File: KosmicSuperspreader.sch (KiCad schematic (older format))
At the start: 27 parts

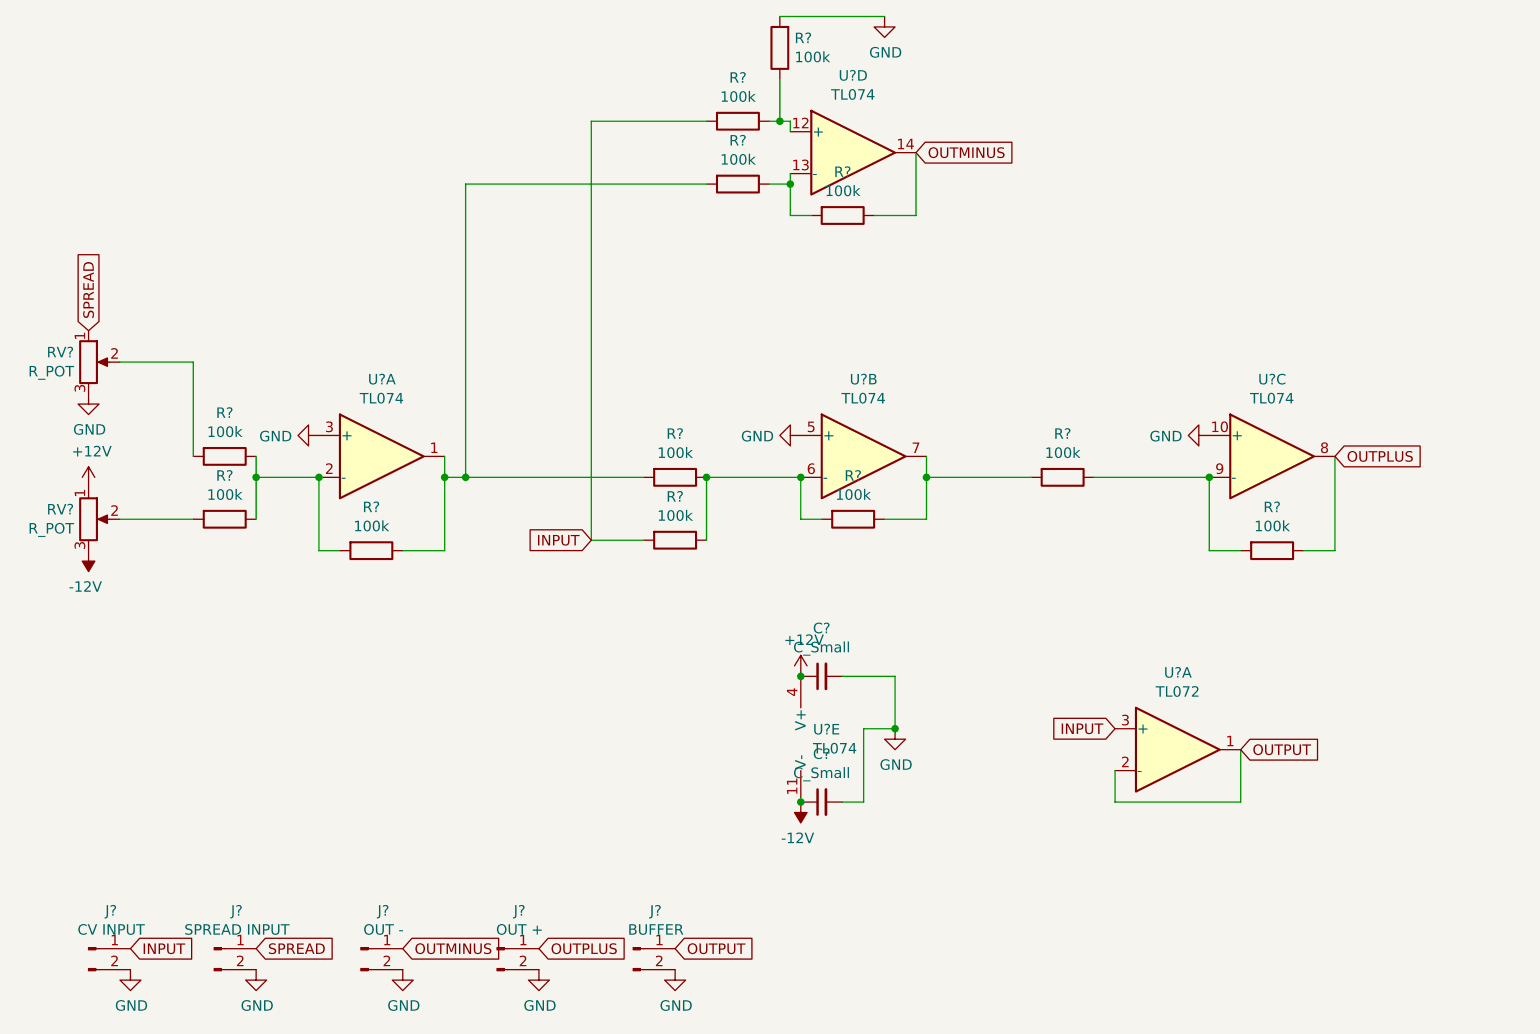
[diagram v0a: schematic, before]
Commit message: Power...
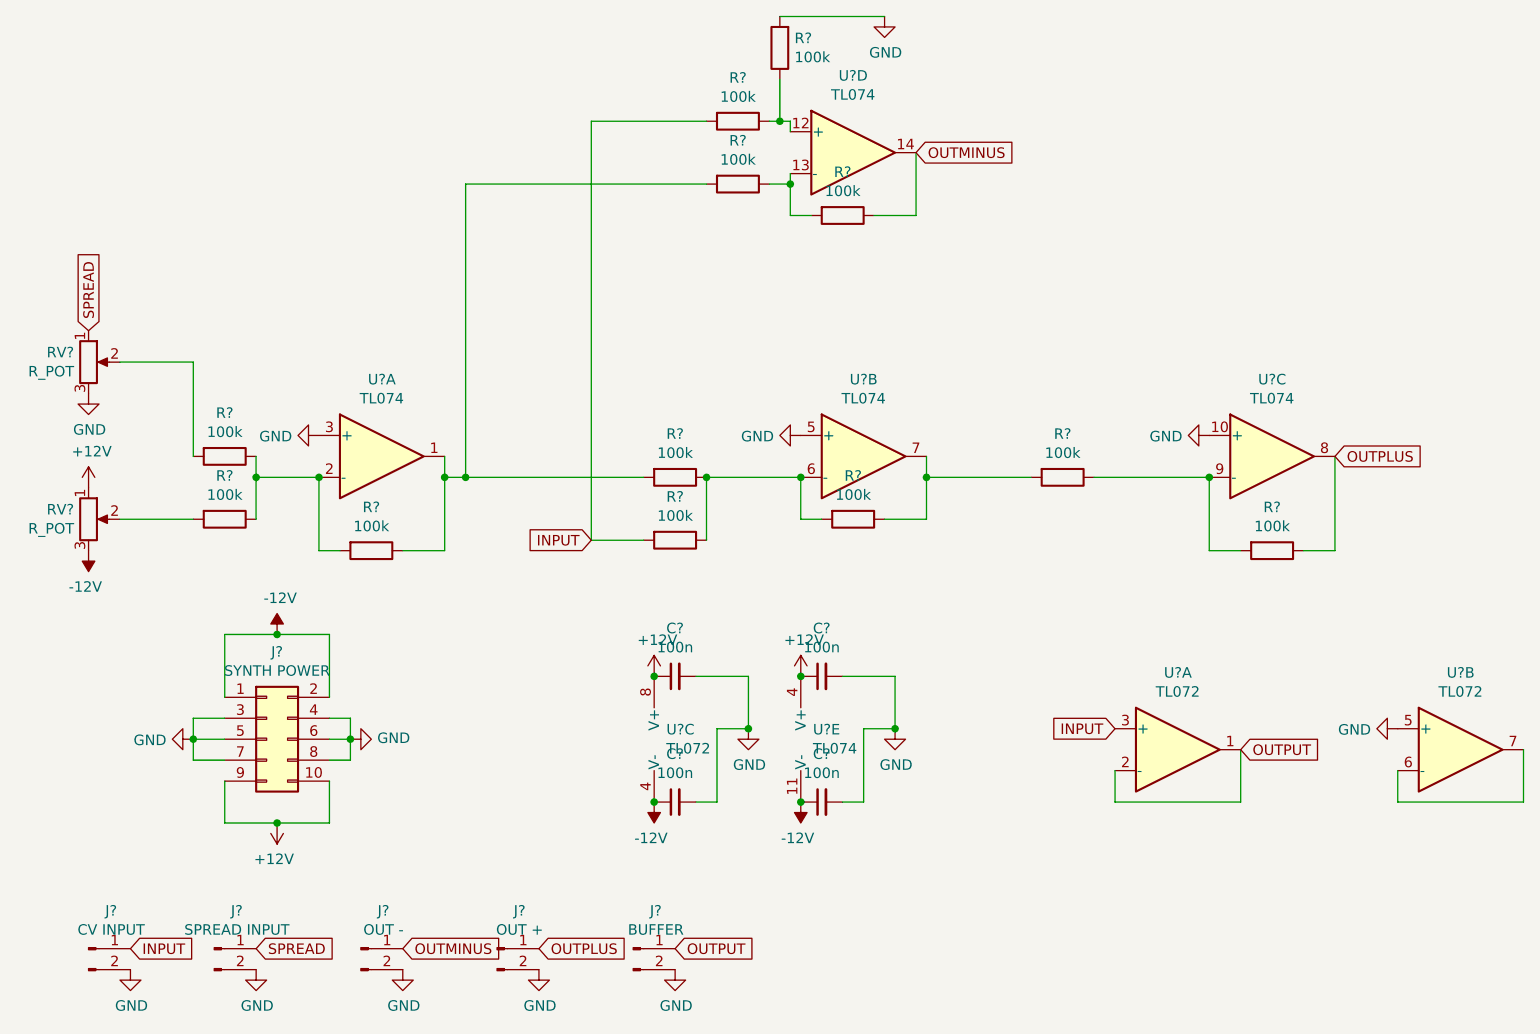
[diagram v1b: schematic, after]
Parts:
- added C? (x2): 100n, symbol Device:C_Small
- added J?: SYNTH POWER, symbol Connector_Generic:Conn_02x05_Odd_Even
- added U? (x2): TL072, symbol Amplifier_Operational:TL072
- C? (x2): value C_Small -> 100n
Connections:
- net +12V: now also C?.1, J?.10 (Pin_10), J?.9 (Pin_9), U?.8 (V+)
- net -12V: now also C?.1, J?.1 (Pin_1), J?.2 (Pin_2), U?.4 (V-)
- net GND: now also C?.2, C?.2, J?.3 (Pin_3), J?.4 (Pin_4), J?.5 (Pin_5), J?.6 (Pin_6), J?.7 (Pin_7), J?.8 (Pin_8), U?.5 (+)
- new net: U?.6 (-), U?.7
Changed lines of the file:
@@
 P 5100 5050
 F 0 "C?" V 5329 5050 50  0000 C CNN
-F 1 "C_Small" V 5238 5050 50  0000 C CNN
+F 1 "100n" V 5238 5050 50  0000 C CNN
 F 2 "" H 5100 5050 50  0001 C CNN
 F 3 "~" H 5100 5050 50  0001 C CNN
@@
 P 5100 5650
 F 0 "C?" V 5329 5650 50  0000 C CNN
-F 1 "C_Small" V 5238 5650 50  0000 C CNN
+F 1 "100n" V 5238 5650 50  0000 C CNN
 F 2 "" H 5100 5650 50  0001 C CNN
 F 3 "~" H 5100 5650 50  0001 C CNN
@@
 	5300 5300 5450 5300
 Connection ~ 5450 5300
+$Comp
+L Amplifier_Operational:TL072 U?
+U 2 1 60B4F880
+P 8150 5400
+F 0 "U?" H 8150 5767 50  0000 C CNN
+F 1 "TL072" H 8150 5676 50  0000 C CNN
+F 2 "" H 8150 5400 50  0001 C CNN
+F 3 "http://www.ti.com/lit/ds/symlink/tl071.pdf" H 8150 5400 50  0001 C CNN
+	2    8150 5400
+	1    0    0    -1
+$EndComp
+Wire Wire Line
+	8450 5400 8450 5650
+Wire Wire Line
+	8450 5650 7850 5650
+Wire Wire Line
+	7850 5650 7850 5500
+$Comp
+L power:GND #PWR?
+U 1 1 60B5124B
+P 7850 5300
+F 0 "#PWR?" H 7850 5050 50  0001 C CNN
+F 1 "GND" V 7855 5172 50  0000 R CNN
+F 2 "" H 7850 5300 50  0001 C CNN
+F 3 "" H 7850 5300 50  0001 C CNN
+	1    7850 5300
+	0    1    1    0
+$EndComp
+$Comp
+L power:+12V #PWR?
+U 1 1 60B520AE
+P 4300 5050
+F 0 "#PWR?" H 4300 4900 50  0001 C CNN
+F 1 "+12V" H 4315 5223 50  0000 C CNN
+F 2 "" H 4300 5050 50  0001 C CNN
+F 3 "" H 4300 5050 50  0001 C CNN
+	1    4300 5050
+	1    0    0    -1
+$EndComp
+$Comp
+L power:-12V #PWR?
+U 1 1 60B520B8
+P 4300 5650
+F 0 "#PWR?" H 4300 5750 50  0001 C CNN
+F 1 "-12V" H 4315 5823 50  0000 C CNN
+F 2 "" H 4300 5650 50  0001 C CNN
+F 3 "" H 4300 5650 50  0001 C CNN
+	1    4300 5650
+	-1   0    0    1
+$EndComp
+$Comp
+L Device:C_Small C?
+U 1 1 60B520C2
+P 4400 5050
+F 0 "C?" V 4629 5050 50  0000 C CNN
+F 1 "100n" V 4538 5050 50  0000 C CNN
+F 2 "" H 4400 5050 50  0001 C CNN
+F 3 "~" H 4400 5050 50  0001 C CNN
+	1    4400 5050
+	0    -1   -1   0
+$EndComp
+$Comp
+L Device:C_Small C?
+U 1 1 60B520CD
+P 4400 5650
+F 0 "C?" V 4629 5650 50  0000 C CNN
+F 1 "100n" V 4538 5650 50  0000 C CNN
+F 2 "" H 4400 5650 50  0001 C CNN
+F 3 "~" H 4400 5650 50  0001 C CNN
+	1    4400 5650
+	0    -1   -1   0
+$EndComp
+$Comp
+L power:GND #PWR?
+U 1 1 60B520D8
+P 4750 5300
+F 0 "#PWR?" H 4750 5050 50  0001 C CNN
+F 1 "GND" H 4755 5127 50  0000 C CNN
+F 2 "" H 4750 5300 50  0001 C CNN
+F 3 "" H 4750 5300 50  0001 C CNN
+	1    4750 5300
+	1    0    0    -1
+$EndComp
+Wire Wire Line
+	4500 5050 4750 5050
+Wire Wire Line
+	4750 5050 4750 5300
+Wire Wire Line
+	4500 5650 4600 5650
+Wire Wire Line
+	4600 5650 4600 5300
+Wire Wire Line
+	4600 5300 4750 5300
+Connection ~ 4750 5300
+$Comp
+L Amplifier_Operational:TL072 U?
+U 3 1 60B54907
+P 4400 5350
+F 0 "U?" H 4358 5396 50  0000 L CNN
+F 1 "TL072" H 4358 5305 50  0000 L CNN
+F 2 "" H 4400 5350 50  0001 C CNN
+F 3 "http://www.ti.com/lit/ds/symlink/tl071.pdf" H 4400 5350 50  0001 C CNN
+	3    4400 5350
+	1    0    0    -1
+$EndComp
+Connection ~ 4300 5650
+Connection ~ 4300 5050
+$Comp
+L Connector_Generic:Conn_02x05_Odd_Even J?
+U 1 1 60B55BA7
+P 2450 5350
+F 0 "J?" H 2500 5767 50  0000 C CNN
+F 1 "SYNTH POWER" H 2500 5676 50  0000 C CNN
+F 2 "" H 2450 5350 50  0001 C CNN
+F 3 "~" H 2450 5350 50  0001 C CNN
+	1    2450 5350
+	1    0    0    -1
+$EndComp
+$Comp
+L power:+12V #PWR?
+U 1 1 60B56459
+P 2500 5750
+F 0 "#PWR?" H 2500 5600 50  0001 C CNN
+F 1 "+12V" H 2515 5923 50  0000 C CNN
+F 2 "" H 2500 5750 50  0001 C CNN
+F 3 "" H 2500 5750 50  0001 C CNN
+	1    2500 5750
+	-1   0    0    1
+$EndComp
+$Comp
+L power:-12V #PWR?
+U 1 1 60B57093
+P 2500 4850
+F 0 "#PWR?" H 2500 4950 50  0001 C CNN
+F 1 "-12V" H 2515 5023 50  0000 C CNN
+F 2 "" H 2500 4850 50  0001 C CNN
+F 3 "" H 2500 4850 50  0001 C CNN
+	1    2500 4850
+	1    0    0    -1
+$EndComp
+Wire Wire Line
+	2750 5150 2750 4850
+Wire Wire Line
+	2750 4850 2500 4850
+Wire Wire Line
+	2500 4850 2250 4850
+Wire Wire Line
+	2250 4850 2250 5150
+Connection ~ 2500 4850
+Wire Wire Line
+	2750 5550 2750 5750
+Wire Wire Line
+	2750 5750 2500 5750
+Wire Wire Line
+	2250 5550 2250 5750
+Wire Wire Line
+	2250 5750 2500 5750
+Connection ~ 2500 5750
+$Comp
+L power:GND #PWR?
+U 1 1 60B5DFE3
+P 2850 5350
+F 0 "#PWR?" H 2850 5100 50  0001 C CNN
+F 1 "GND" V 2855 5222 50  0000 R CNN
+F 2 "" H 2850 5350 50  0001 C CNN
+F 3 "" H 2850 5350 50  0001 C CNN
+	1    2850 5350
+	0    -1   -1   0
+$EndComp
+Wire Wire Line
+	2750 5250 2850 5250
+Wire Wire Line
+	2850 5250 2850 5350
+Wire Wire Line
+	2750 5350 2850 5350
+Connection ~ 2850 5350
+Wire Wire Line
+	2750 5450 2850 5450
+Wire Wire Line
+	2850 5450 2850 5350
+$Comp
+L power:GND #PWR?
+U 1 1 60B63CE1
+P 2100 5350
+F 0 "#PWR?" H 2100 5100 50  0001 C CNN
+F 1 "GND" V 2105 5222 50  0000 R CNN
+F 2 "" H 2100 5350 50  0001 C CNN
+F 3 "" H 2100 5350 50  0001 C CNN
+	1    2100 5350
+	0    1    1    0
+$EndComp
+Wire Wire Line
+	2250 5250 2100 5250
+Wire Wire Line
+	2100 5250 2100 5350
+Wire Wire Line
+	2250 5350 2100 5350
+Connection ~ 2100 5350
+Wire Wire Line
+	2250 5450 2100 5450
+Wire Wire Line
+	2100 5450 2100 5350
 $EndSCHEMATC
